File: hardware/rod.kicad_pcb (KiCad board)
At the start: 2 copper layers, 10 parts, among them P1 arduino_mini, P2 arduino_mini, P4 DOTSTAR, P5 USB_B, SW1 SW_PUSH_R, SW2 SW_PUSH_B, SW3 SW_PUSH_G

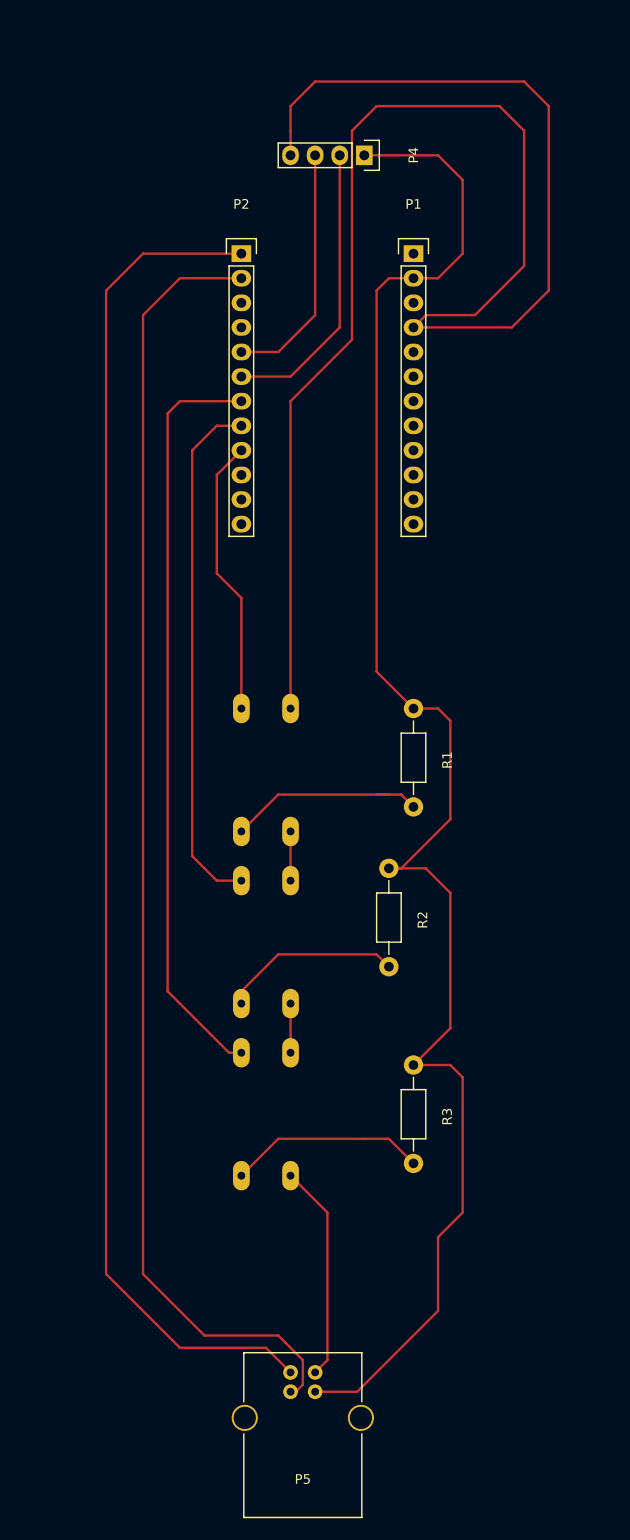
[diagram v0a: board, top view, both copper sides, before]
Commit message: "Updated PCB"
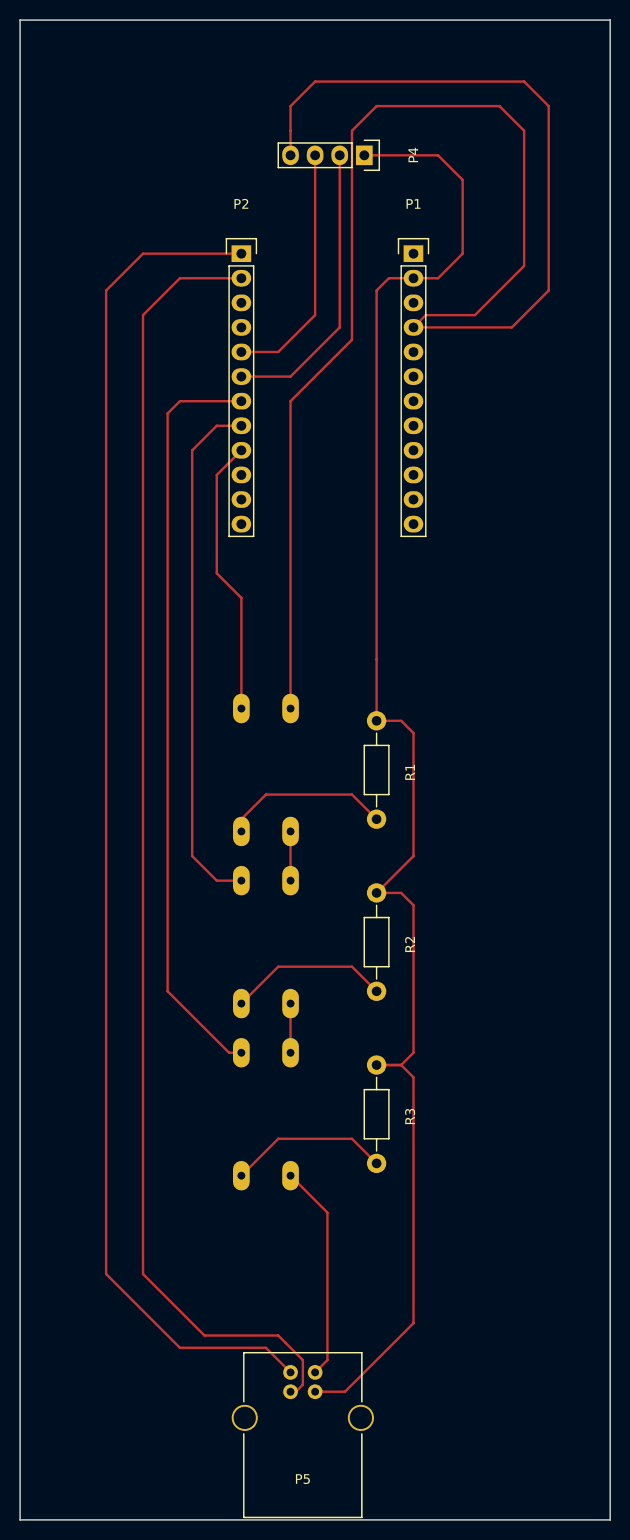
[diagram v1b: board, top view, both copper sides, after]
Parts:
- moved R1 4.02 mm to (115.6, 108.0)
- moved R3 3.81 mm to (115.6, 143.5)
- moved R2 2.84 mm to (115.6, 125.7)
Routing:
- net GND: track 170.7 -> 162.9 mm
- net 6: track 51.2 -> 46.1 mm
- net 4: track 98.5 -> 94.7 mm
- net 5: track 72.8 -> 72.0 mm
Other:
- board outline added: 61 x 154.9 mm
